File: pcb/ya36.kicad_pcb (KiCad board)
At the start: 2 copper layers, 224.5 x 67 mm, 78 parts, among them J1 MJ-4PP-9, J2 MJ-4PP-9, SW1 SW_PUSH, SW10 SW_PUSH, SW11 SW_PUSH, SW12 SW_PUSH, SW13 SW_PUSH, SW14 SW_PUSH, SW15 SW_PUSH, SW16 SW_PUSH, SW17 SW_PUSH, SW18 SW_PUSH, SW19 SW_PUSH, SW2 SW_PUSH, SW20 SW_PUSH, SW21 SW_PUSH, SW22 SW_PUSH, SW23 SW_PUSH, SW24 SW_PUSH, SW25 SW_PUSH, SW26 SW_PUSH, SW27 SW_PUSH, SW28 SW_PUSH, SW29 SW_PUSH, SW3 SW_PUSH, SW30 SW_PUSH, SW31 SW_PUSH, SW32 SW_PUSH, SW33 SW_PUSH, SW34 SW_PUSH, SW35 SW_PUSH, SW36 SW_PUSH, SW4 SW_PUSH, SW5 SW_PUSH, SW6 SW_PUSH, SW7 SW_PUSH, SW8 SW_PUSH, SW9 SW_PUSH, U1 ProMicro, U2 ProMicro

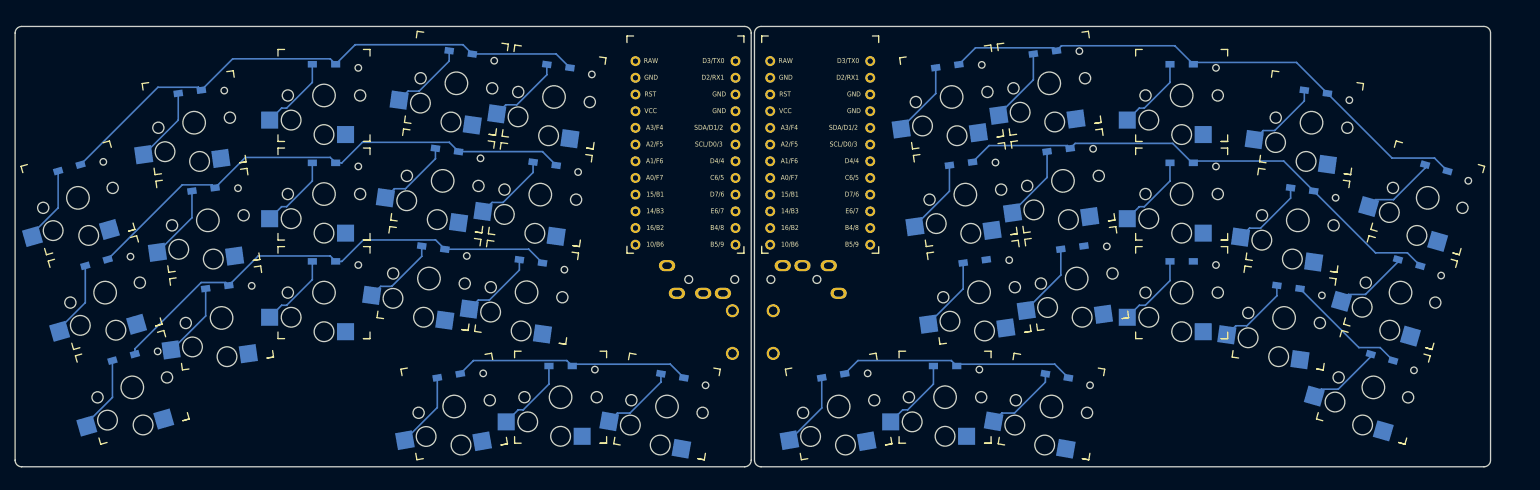
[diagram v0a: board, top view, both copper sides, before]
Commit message: Update route
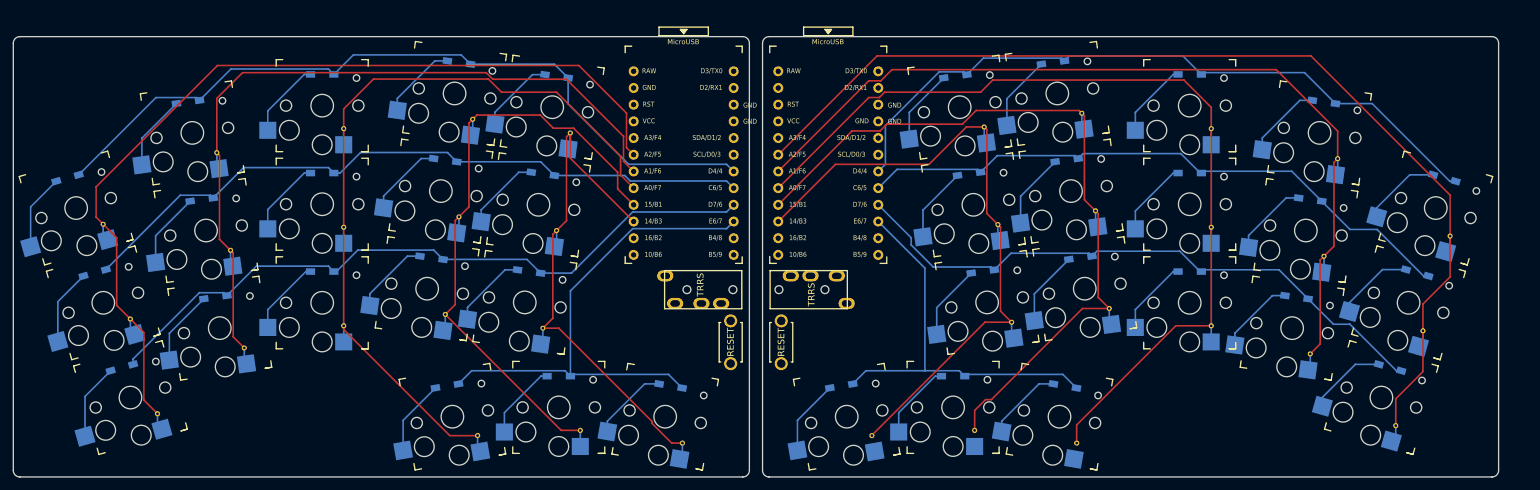
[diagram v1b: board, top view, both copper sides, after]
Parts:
- moved SW36 1.98 mm to (161.5, 111.4)
- moved SW22 1.98 mm to (193.6, 62.2)
- moved D19 1.98 mm to (252.5, 75.1)
- moved D27 1.98 mm to (195.0, 72.3)
- moved D33 1.98 mm to (182.2, 89.3)
- moved SW24 1.98 mm to (247.0, 94.0)
- moved SW28 1.98 mm to (180.8, 79.1)
- moved D28 1.98 mm to (180.2, 74.4)
- moved D30 1.98 mm to (230.0, 93.2)
- moved D32 1.98 mm to (197.1, 87.2)
- moved SW33 1.98 mm to (182.9, 94.0)
- moved SW34 1.98 mm to (193.9, 111.4)
- moved D23 1.98 mm to (178.1, 59.6)
- moved D20 1.98 mm to (234.1, 63.5)
- moved D21 1.98 mm to (213.7, 59.3)
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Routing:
- net COL5R: track 0.00 -> 163.6 mm
- net COL3R: track 0.00 -> 144.5 mm
- net COL1: track 0.00 -> 144.4 mm
- net COL4R: track 0.00 -> 138.7 mm
- net COL3: track 0.00 -> 125.1 mm
- net COL2R: track 0.00 -> 121.4 mm
- net COL2: track 0.00 -> 120.9 mm
- net COL1R: track 0.00 -> 104.9 mm
- net COL4: track 0.00 -> 101.3 mm
- net COL5: track 0.00 -> 87.8 mm
- net ROW3R: track 18.7 -> 93.6 mm
- net ROW4: track 36.2 -> 78.4 mm
- net ROW3: track 72.2 -> 105.9 mm
- net ROW1: track 84.5 -> 117.9 mm
- net ROW2: track 78.1 -> 106.2 mm
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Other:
- board size 224.5 x 67 mm -> 226 x 67 mm

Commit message: Update pcb
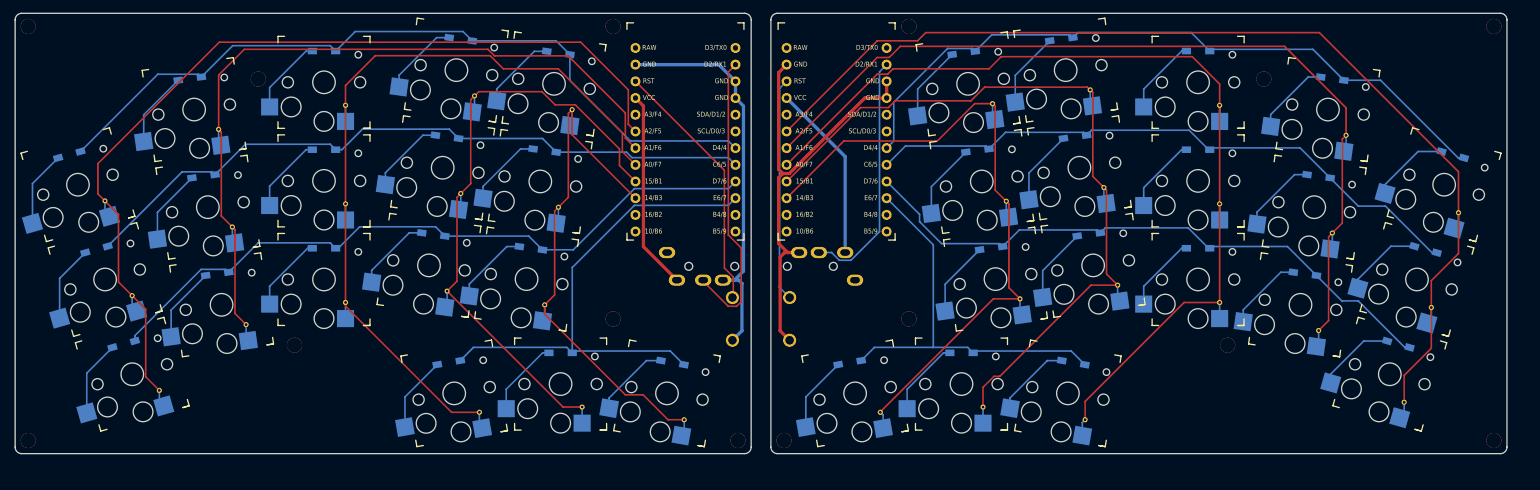
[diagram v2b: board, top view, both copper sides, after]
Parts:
- added Ref**: Val**, kbd:M2_Threads_v2, F.Cu at (260.0, 52.0)
- added Ref**: Val**, kbd:M2_Threads_v2, F.Cu at (77.5, 100.5)
- added Ref**: Val**, kbd:M2_Threads_v2, F.Cu at (126.0, 52.0)
- added Ref**: Val**, kbd:M2_Threads_v2, F.Cu at (37.0, 52.0)
- added Ref**: Val**, kbd:M2_Threads_v2, F.Cu at (37.0, 115.0)
- added Ref**: Val**, kbd:M2_Threads_v2, F.Cu at (145.0, 115.0)
- added Ref**: Val**, kbd:M2_Threads_v2, F.Cu at (260.0, 115.0)
- added Ref**: Val**, kbd:M2_Threads_v2, F.Cu at (152.0, 115.0)
- added Ref**: Val**, kbd:M2_Threads_v2, F.Cu at (219.5, 100.5)
- added Ref**: Val**, kbd:M2_Threads_v2, F.Cu at (171.0, 96.5)
- added Ref**: Val**, kbd:M2_Threads_v2, F.Cu at (225.0, 60.0)
- added Ref**: Val**, kbd:M2_Threads_v2, F.Cu at (171.0, 52.0)
- added Ref**: Val**, kbd:M2_Threads_v2, F.Cu at (72.0, 60.0)
- added Ref**: Val**, kbd:M2_Threads_v2, F.Cu at (126.0, 96.5)
- moved D28 3.77 mm to (181.4, 70.9)
- moved D30 3.77 mm to (231.2, 89.7)
- moved D32 3.77 mm to (198.4, 83.7)
- moved SW33 3.77 mm to (184.2, 90.4)
- moved SW34 3.77 mm to (195.2, 107.8)
- moved D23 3.77 mm to (179.3, 56.0)
- moved SW36 3.77 mm to (162.8, 107.8)
- moved D20 3.77 mm to (235.4, 59.9)
- moved D21 3.77 mm to (215.0, 55.8)
- moved D22 3.77 mm to (194.2, 53.9)
- moved D24 3.77 mm to (249.6, 85.9)
- moved D25 3.77 mm to (233.3, 74.8)
- moved D26 3.77 mm to (215.0, 70.8)
- moved D29 3.77 mm to (245.5, 100.4)
- moved D31 3.77 mm to (215.0, 85.8)
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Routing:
- net GND1: track 0.00 -> 69.7 mm
- net GND: track 0.00 -> 61.0 mm
- net DATA: track 0.00 -> 45.1 mm
- net RESET: track 0.00 -> 39.1 mm
- net DATAR: track 0.00 -> 37.4 mm
- net RESETR: track 0.00 -> 34.0 mm
- net VCC: track 0.00 -> 30.3 mm
- net VDD: track 0.00 -> 27.2 mm
- net COL3R: track 144.5 -> 147.1 mm
- net COL1R: track 104.9 -> 107.5 mm
- net COL2R: track 121.4 -> 123.8 mm
- net COL5: track 87.8 -> 88.5 mm
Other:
- board size 226 x 67 mm -> 227 x 67 mm

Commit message: Update pcb
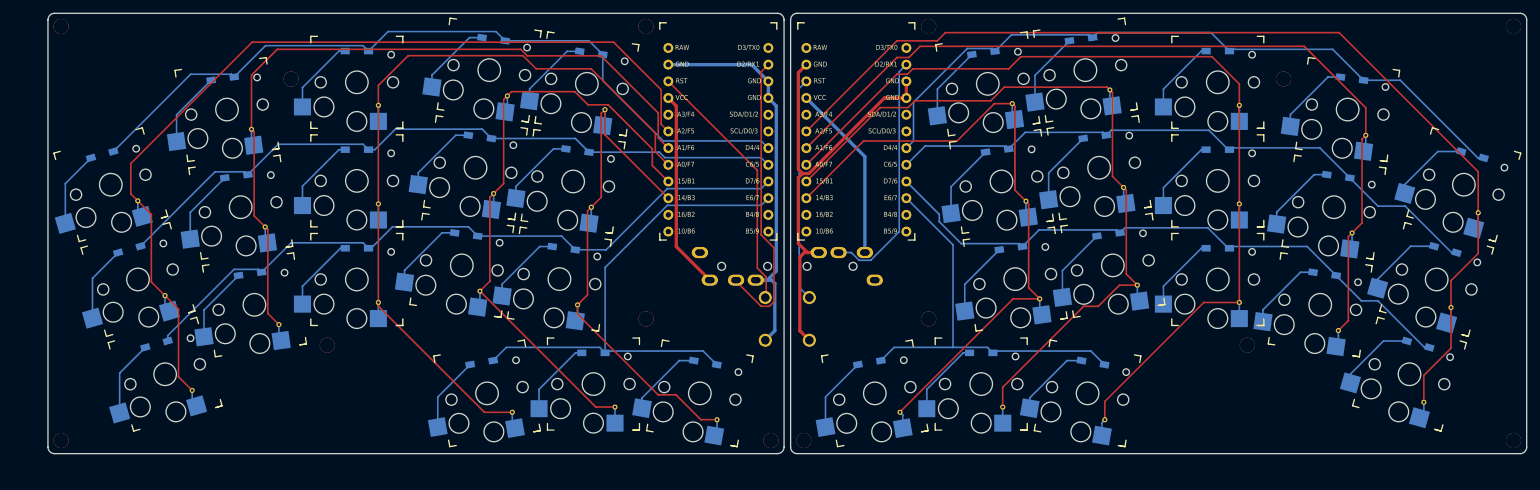
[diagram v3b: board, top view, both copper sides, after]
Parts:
- moved D1 5.00 mm to (48.3, 71.5)
- moved D10 5.00 mm to (120.6, 70.9)
- moved D11 5.00 mm to (56.5, 100.4)
- moved D12 5.00 mm to (70.8, 89.7)
- moved D13 5.00 mm to (87.0, 85.8)
- moved D14 5.00 mm to (103.6, 83.7)
- moved D15 5.00 mm to (118.5, 85.7)
- moved D16 5.00 mm to (106.0, 103.2)
- moved D17 5.00 mm to (123.0, 101.7)
- moved D18 5.00 mm to (140.0, 103.2)
- moved D2 5.00 mm to (66.6, 59.9)
- moved D3 5.00 mm to (87.0, 55.8)
- moved D4 5.00 mm to (107.8, 53.9)
- moved D5 5.00 mm to (122.7, 56.0)
- moved D6 5.00 mm to (52.4, 85.9)
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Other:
- board size 227 x 67 mm -> 225 x 67 mm
